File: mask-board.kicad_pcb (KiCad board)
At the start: 2 copper layers, 51.8 x 31.8 mm, 60 parts, among them J1 SWIM Connector, J2 I2C Breakout, M1 Fan_3pin, M2 Fan_3pin, M3 Motor_DC, Q1 DMN10H220L, Q2 DMN10H220L, Q3 DMN10H220L, Q4 DMN10H220L, SW1 SW_Push, U1 STM8S003F3P, U2 TLV77333PDBVR, U3 SGP40-D-R4

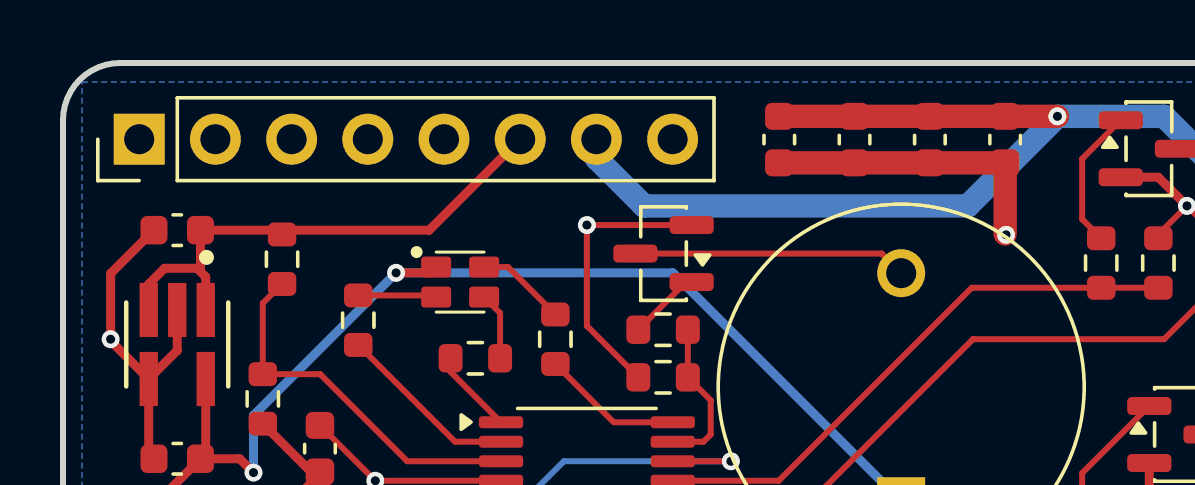
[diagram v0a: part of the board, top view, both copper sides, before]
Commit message: Generate gerbers
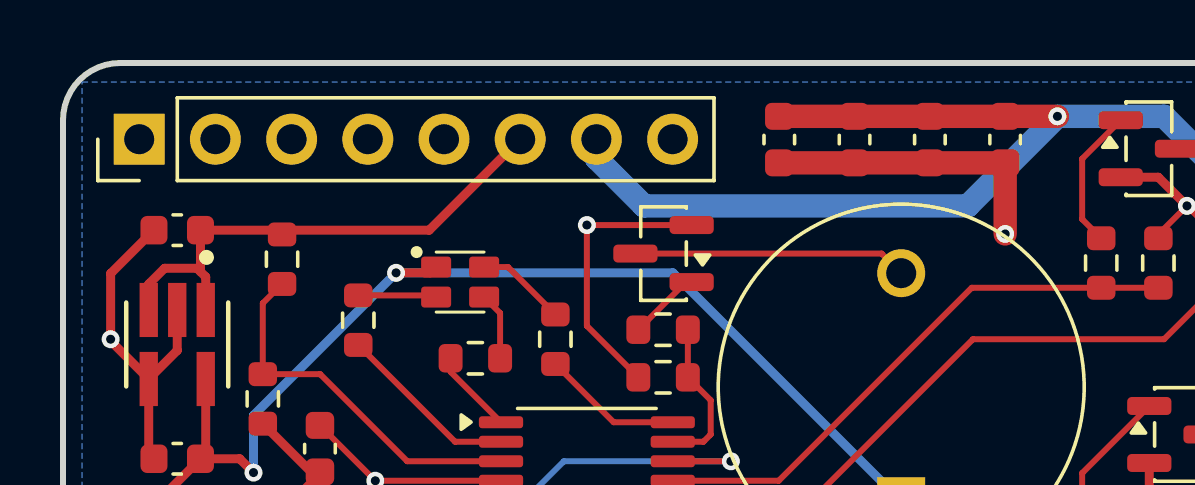
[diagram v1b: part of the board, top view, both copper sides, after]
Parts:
- A1: moved to B.Cu
- turned A1 to -90 degrees
